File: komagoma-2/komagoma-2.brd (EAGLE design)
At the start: 34 x 42 mm, 16 parts, among them IC1 TB6612FNGSSOP24, U1 XIAO-ESP32C3A

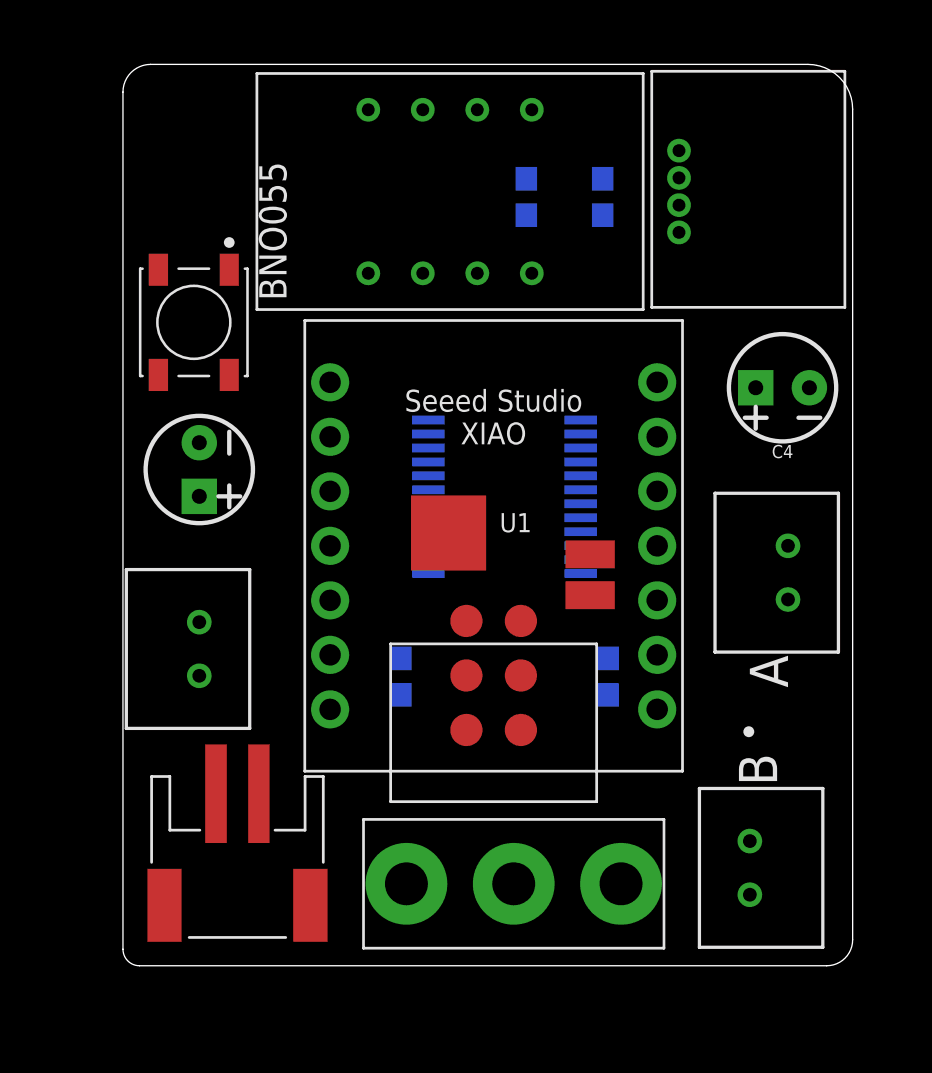
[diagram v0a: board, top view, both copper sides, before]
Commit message: order : .brd
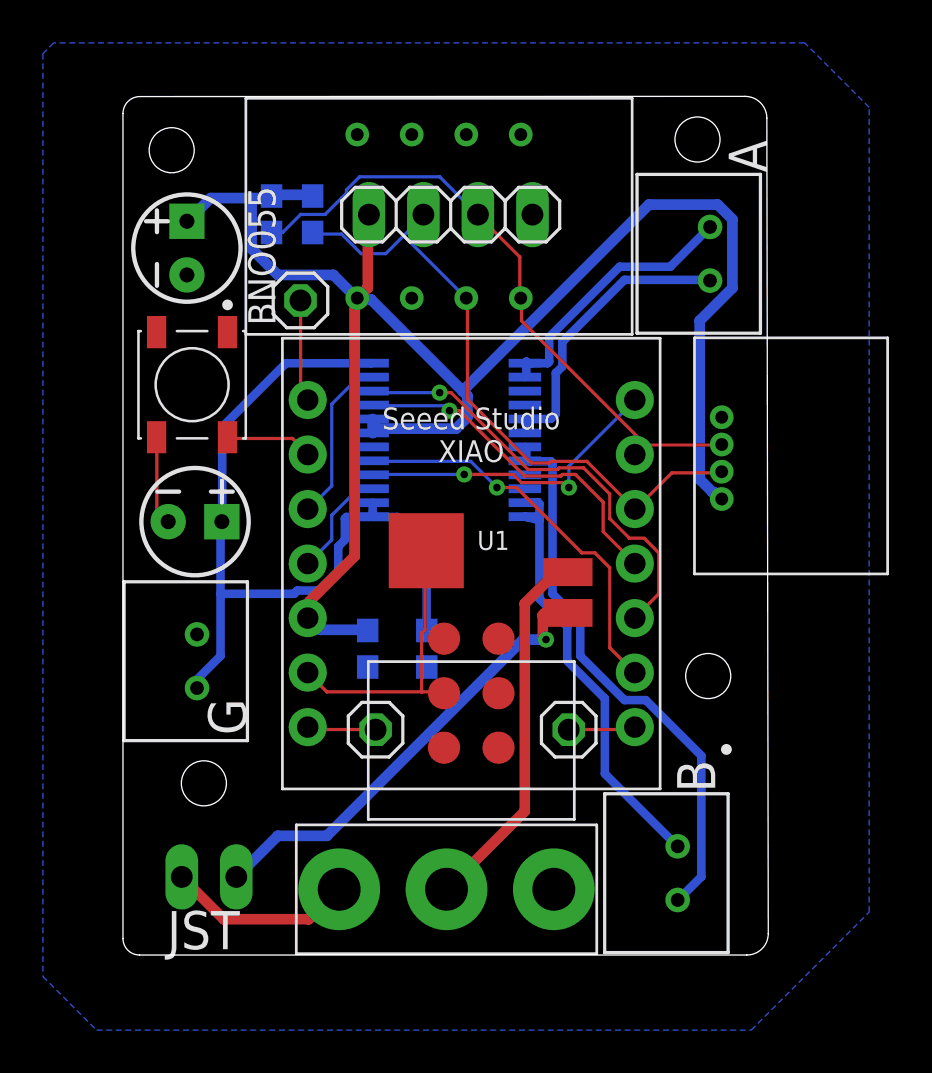
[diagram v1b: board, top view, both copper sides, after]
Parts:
- added 5V, A0, D7: PINHD-1X1, Connector:1X01
- added X1: JST-XH-02-PIN-LONG-PAD, Rembrandt Electronics - JST XH Connectors v1-0:JST-XH-02-PACKAGE-LONG-PAD
- JP1: value JSTPH2 -> PINHD-1X4; device Tutorial - Fusion 360:JSTPH2 -> Connector:1X04
- moved JP1 32.3 mm to (14.0, 35.5), turned to 0 degrees
- moved C4 28.5 mm to (1.71, 33.9), turned to 90 degrees
- moved XH 15.3 mm to (26.1, 34.9)
- moved R1 13.5 mm to (7.57, 35.5)
- moved U$2 12.6 mm to (26.6, 24.2)
- moved R2 11.9 mm to (5.65, 35.5)
- moved C2 8.55 mm to (12.9, 15.3)
- moved XH1 4.05 mm to (24.6, 6.06), turned to 270 degrees
- moved IC1 3.71 mm to (13.9, 25.0)
- moved CONNECTOR1 3.14 mm to (8.81, 4.06)
- moved D1 2.91 mm to (1.95, 27.6)
- moved C1 2.44 mm to (2.09, 21.2), turned to 0 degrees
- moved C3 2.02 mm to (10.1, 15.3)
- moved U1 1.33 mm to (15.0, 19.2)
- moved U$1 1.27 mm to (13.5, 35.4)
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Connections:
- new net 5V: 5V.1, U1.P$14
- new net A0: A0.1, U1.P$1
- new net D7: D7.1, U1.P$8
- net +3V3: now also JP1.1
- net BAT-: now also X1.2; no longer JP1.1
- net BATT: now also X1.1; no longer JP1.2
- net GND: now also JP1.4
- net SCL: now also JP1.3
- net SDA: now also JP1.2
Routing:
- net +3V3: track 0.00 -> 81.6 mm
- net VM: track 0.00 -> 38.4 mm
- net SCL: track 0.00 -> 30.2 mm
- net SDA: track 0.00 -> 30.0 mm
- net BO2: track 0.00 -> 26.3 mm
- net BAT-: track 0.00 -> 21.4 mm, vias 0 -> 1
- net N$6: track 0.00 -> 20.7 mm, vias 0 -> 1
- net BO1: track 0.00 -> 20.6 mm
- net N$8: track 0.00 -> 18.5 mm, vias 0 -> 1
- net GND: track 0.00 -> 17.6 mm
- net BAT+: track 0.00 -> 17.4 mm
- net N$3: track 0.00 -> 16.2 mm, vias 0 -> 1
- net N$9: track 0.00 -> 14.8 mm, vias 0 -> 2
- net AO2: track 0.00 -> 13.8 mm
- net AO1: track 0.00 -> 12.9 mm
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- added copper zone on layer 16, net GND
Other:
- board size 34 x 42 mm -> 30.1 x 40 mm
- board text added: "G"
- board text added: "JST"
